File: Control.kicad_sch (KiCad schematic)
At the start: 25 parts, among them Q1 MMBT3904, U10 74AHC1G14GW, U11 74AHCT08PW, U12 74AHCT32PW, U13 74AHCT32PW, U15 74AHC1G14GW, U3 74AHCT00PW, U4 74AHC1G14GW, U6 74AHCT02PW, U7 74AHCT08PW, U9 74AHCT08PW

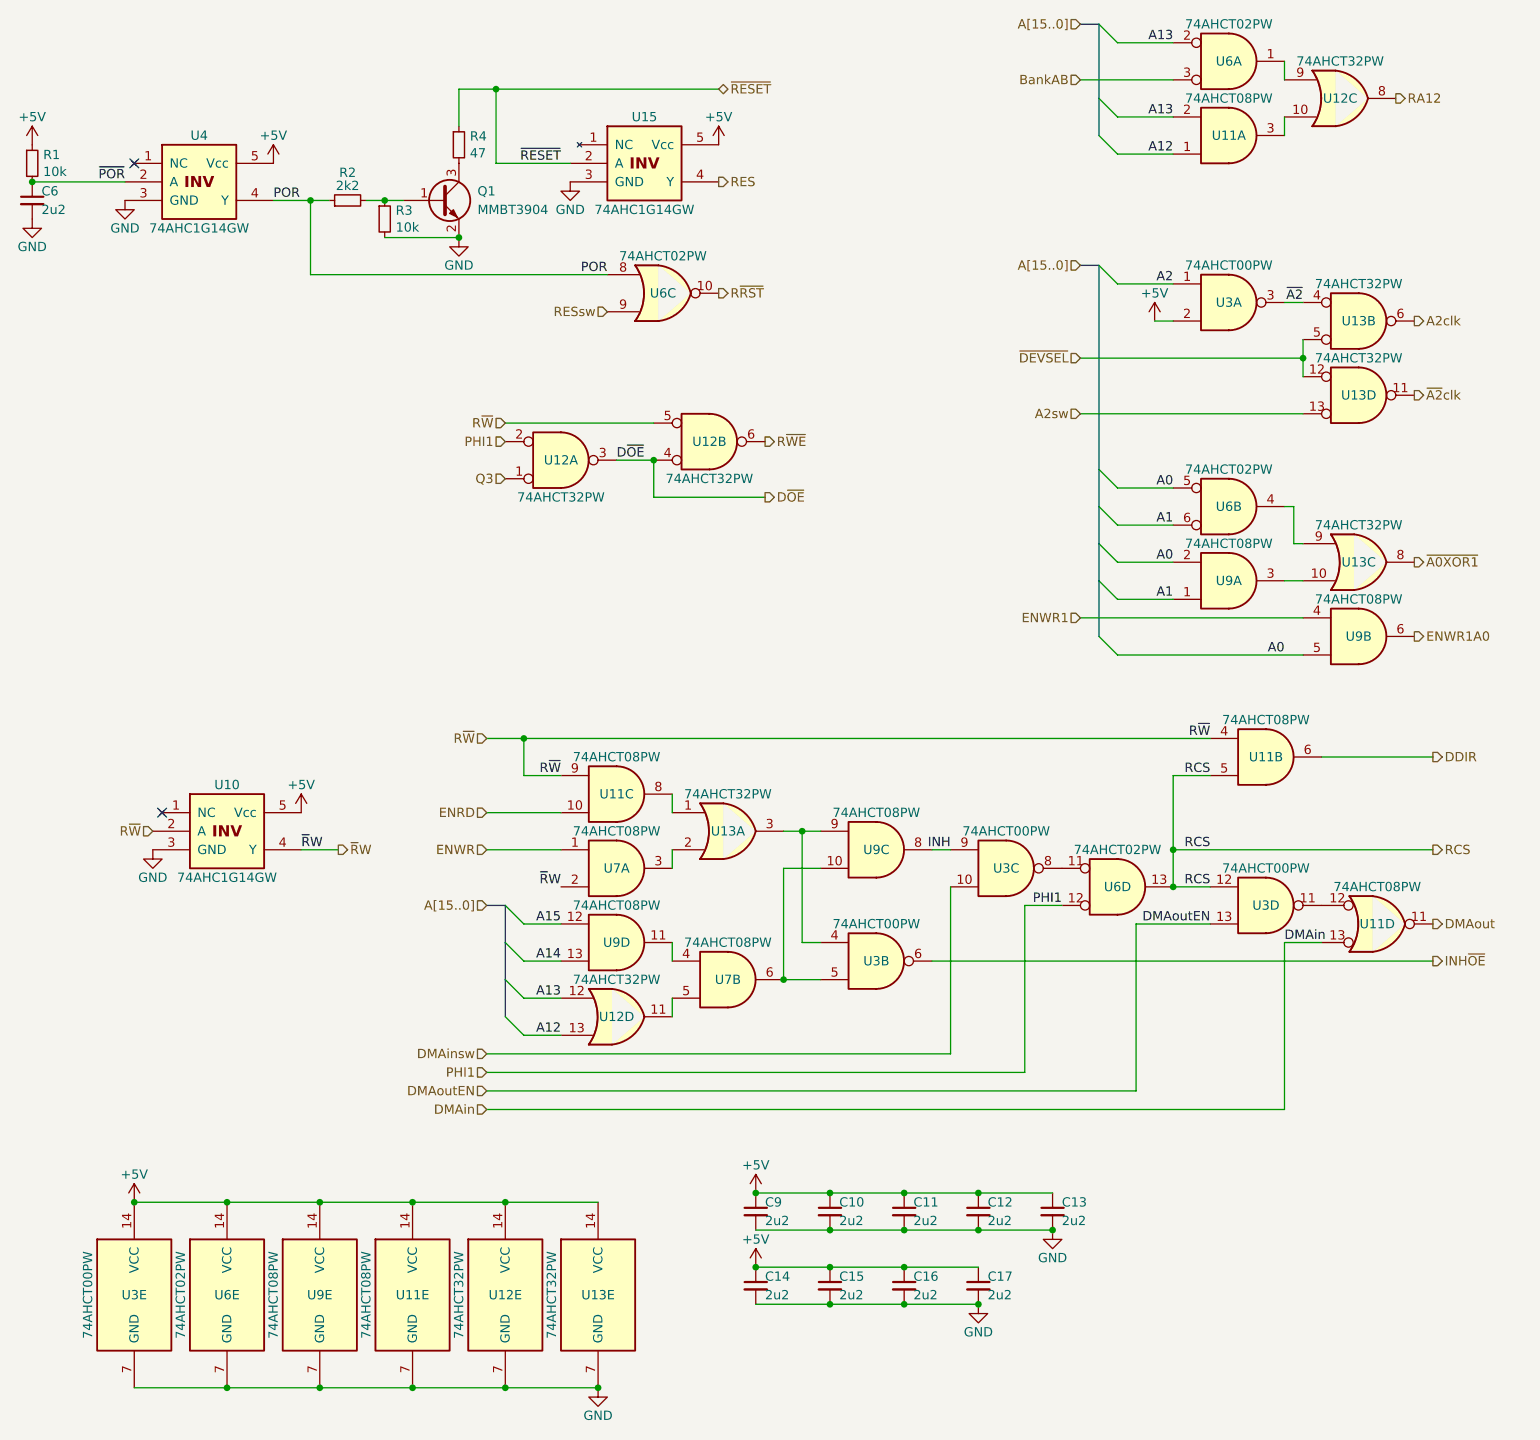
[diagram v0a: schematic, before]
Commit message: more
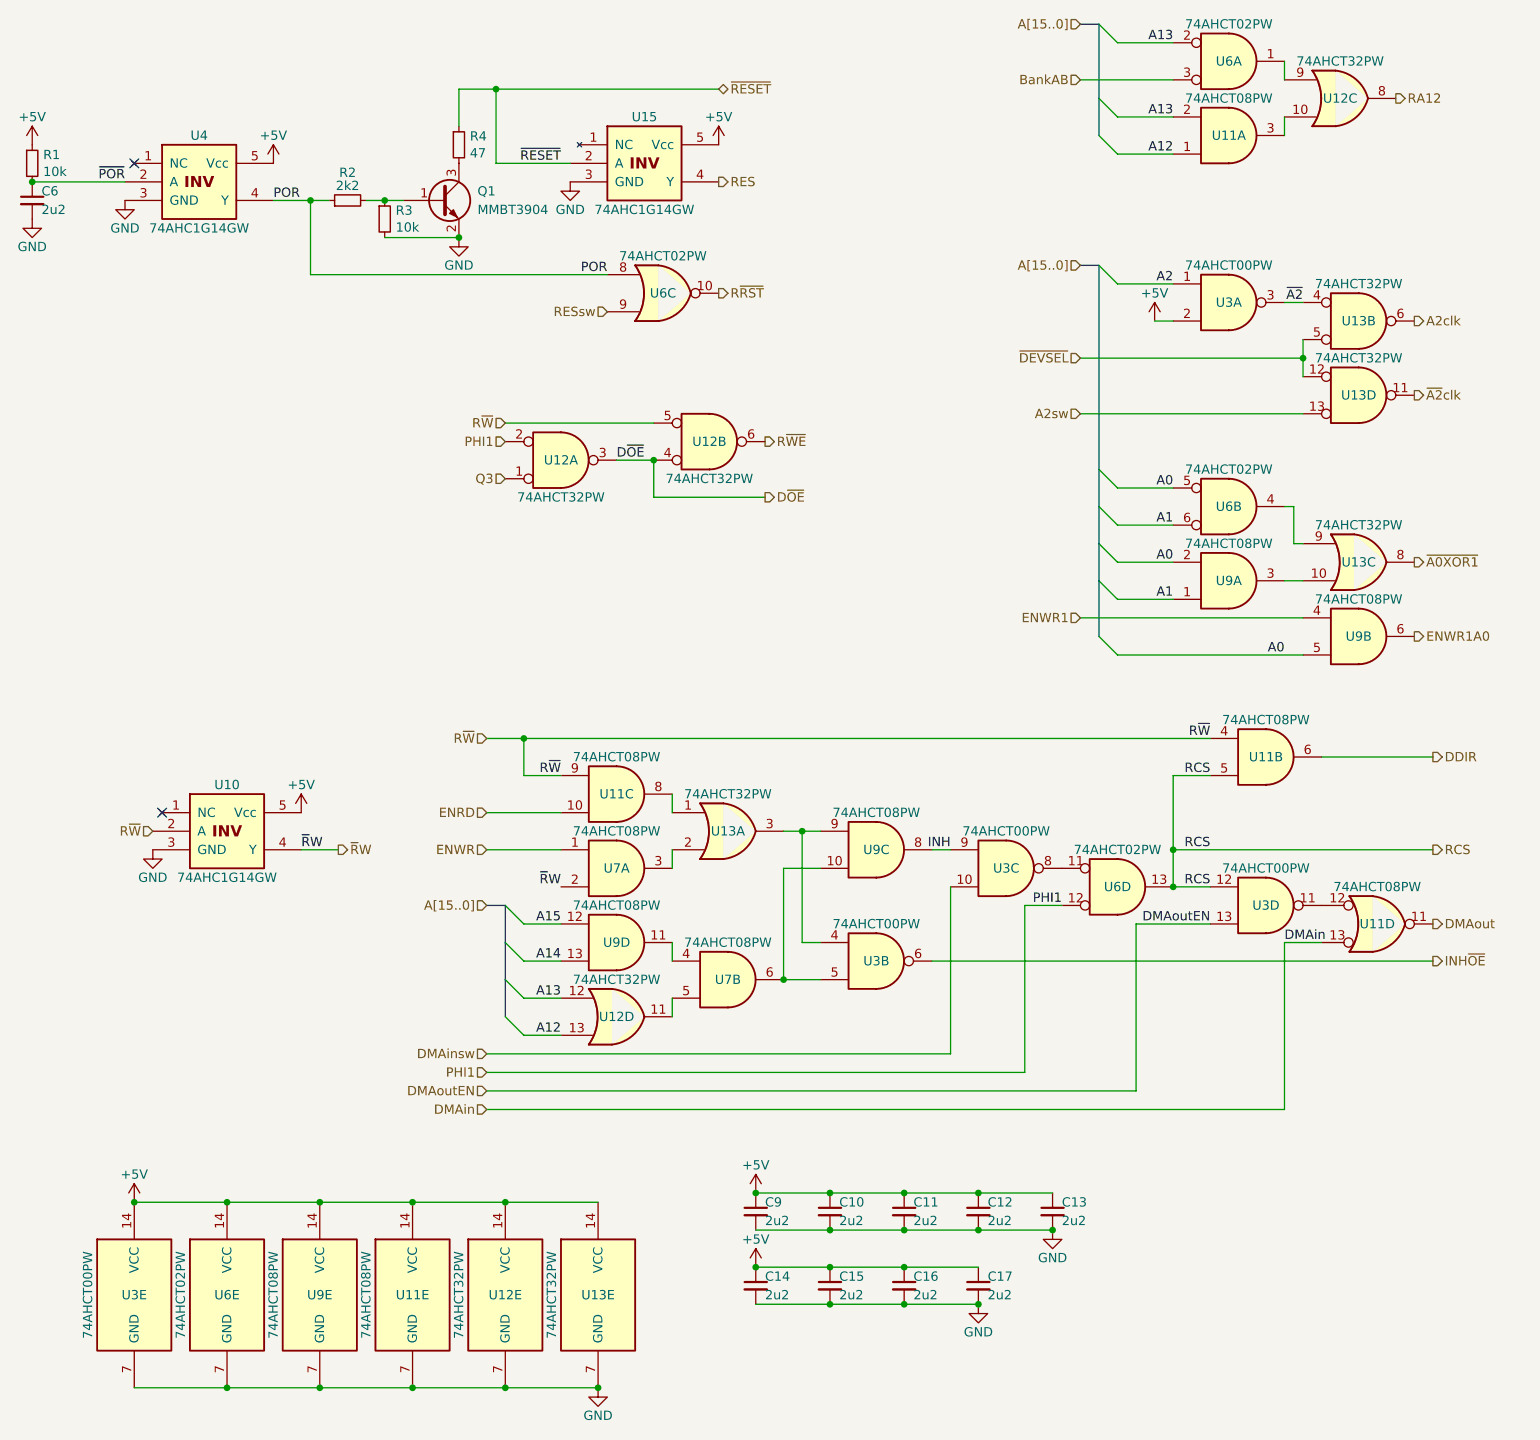
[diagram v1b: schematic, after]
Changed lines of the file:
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@@
 (kicad_sch
-	(version 20231120)
+	(version 20250114)
 	(generator "eeschema")
-	(generator_version "8.0")
+	(generator_version "9.0")
 	(paper "A4")
 	(title_block
@@
 	(label "A1"
 		(at 179.07 74.93 180)
-		(fields_autoplaced yes)
 		(effects
 			(font
@@
 	(label "A12"
 		(at 179.07 24.13 180)
-		(fields_autoplaced yes)
 		(effects
 			(font
@@
 	(label "INH"
 		(at 148.59 119.38 180)
-		(fields_autoplaced yes)
 		(effects
 			(font
@@
 	(label "D~{OE}"
 		(at 102.87 66.04 0)
-		(fields_autoplaced yes)
 		(effects
 			(font
@@
 	(label "A0"
 		(at 179.07 69.85 180)
-		(fields_autoplaced yes)
 		(effects
 			(font
@@
 	(label "~{RESET}"
 		(at 95.25 25.4 180)
-		(fields_autoplaced yes)
 		(effects
 			(font
@@
 	(label "A0"
 		(at 179.07 80.01 180)
-		(fields_autoplaced yes)
 		(effects
 			(font
@@
 	(label "DMAin"
 		(at 194.31 132.08 0)
-		(fields_autoplaced yes)
 		(effects
 			(font
@@
 	(label "A1"
 		(at 179.07 85.09 180)
-		(fields_autoplaced yes)
 		(effects
 			(font
@@
 	(label "DMAoutEN"
 		(at 184.15 129.54 180)
-		(fields_autoplaced yes)
 		(effects
 			(font
@@
 	(label "A0"
 		(at 194.31 92.71 180)
-		(fields_autoplaced yes)
 		(effects
 			(font
@@
 	(label "~{R}W"
 		(at 59.69 119.38 0)
-		(fields_autoplaced yes)
 		(effects
 			(font
@@
 	(label "POR"
 		(at 55.88 30.48 0)
-		(fields_autoplaced yes)
 		(effects
 			(font
@@
 	(label "POR"
 		(at 101.6 40.64 180)
-		(fields_autoplaced yes)
 		(effects
 			(font
@@
 	(label "~{A2}"
 		(at 196.85 44.45 180)
-		(fields_autoplaced yes)
 		(effects
 			(font
@@
 	(label "RCS"
 		(at 184.15 109.22 180)
-		(fields_autoplaced yes)
 		(effects
 			(font
@@
 	(label "~{R}W"
 		(at 95.25 124.46 180)
-		(fields_autoplaced yes)
 		(effects
 			(font
@@
 	(label "A2"
 		(at 179.07 41.91 180)
-		(fields_autoplaced yes)
 		(effects
 			(font
@@
 	(label "A13"
 		(at 179.07 8.89 180)
-		(fields_autoplaced yes)
 		(effects
 			(font
@@
 	(label "PHI1"
 		(at 163.83 127 180)
-		(fields_autoplaced yes)
 		(effects
 			(font
@@
 	(label "A13"
 		(at 95.25 139.7 180)
-		(fields_autoplaced yes)
 		(effects
 			(font
@@
 	(label "A13"
 		(at 179.07 19.05 180)
-		(fields_autoplaced yes)
 		(effects
 			(font
@@
 	(label "A15"
 		(at 95.25 129.54 180)
-		(fields_autoplaced yes)
 		(effects
 			(font
@@
 	(label "~{POR}"
 		(at 35.56 27.94 180)
-		(fields_autoplaced yes)
 		(effects
 			(font
@@
 	(label "A14"
 		(at 95.25 134.62 180)
-		(fields_autoplaced yes)
 		(effects
 			(font
@@
 	(label "R~{W}"
 		(at 184.15 104.14 180)
-		(fields_autoplaced yes)
 		(effects
 			(font
@@
 	(label "RCS"
 		(at 184.15 119.38 180)
-		(fields_autoplaced yes)
 		(effects
 			(font
@@
 	(label "A12"
 		(at 95.25 144.78 180)
-		(fields_autoplaced yes)
 		(effects
 			(font
@@
 	(label "RCS"
 		(at 184.15 124.46 180)
-		(fields_autoplaced yes)
 		(effects
 			(font
@@
 	(label "R~{W}"
 		(at 95.25 109.22 180)
-		(fields_autoplaced yes)
 		(effects
 			(font
@@
 		(shape output)
 		(at 212.09 46.99 0)
-		(fields_autoplaced yes)
 		(effects
 			(font
@@
 		(shape output)
 		(at 212.09 80.01 0)
-		(fields_autoplaced yes)
 		(effects
 			(font
@@
 		(shape input)
 		(at 166.37 13.97 180)
-		(fields_autoplaced yes)
 		(effects
 			(font
@@
 		(shape input)
 		(at 87.63 60.96 180)
-		(fields_autoplaced yes)
 		(effects
 			(font
@@
 		(shape input)
 		(at 166.37 6.35 180)
-		(fields_autoplaced yes)
 		(effects
 			(font
@@
 		(shape output)
 		(at 214.63 129.54 0)
-		(fields_autoplaced yes)
 		(effects
 			(font
@@
 		(shape input)
 		(at 87.63 63.5 180)
-		(fields_autoplaced yes)
 		(effects
 			(font
@@
 		(shape output)
 		(at 64.77 119.38 0)
-		(fields_autoplaced yes)
 		(effects
 			(font
@@
 		(shape input)
 		(at 85.09 119.38 180)
-		(fields_autoplaced yes)
 		(effects
 			(font
@@
 		(shape input)
 		(at 85.09 152.4 180)
-		(fields_autoplaced yes)
 		(effects
 			(font
@@
 		(shape input)
 		(at 166.37 87.63 180)
-		(fields_autoplaced yes)
 		(effects
 			(font
@@
 		(shape input)
 		(at 39.37 116.84 180)
-		(fields_autoplaced yes)
 		(effects
 			(font
@@
 		(shape input)
 		(at 166.37 39.37 180)
-		(fields_autoplaced yes)
 		(effects
 			(font
@@
 		(shape input)
 		(at 85.09 147.32 180)
-		(fields_autoplaced yes)
 		(effects
 			(font
@@
 		(shape input)
 		(at 87.63 68.58 180)
-		(fields_autoplaced yes)
 		(effects
 			(font
@@
 		(shape output)
 		(at 214.63 119.38 0)
-		(fields_autoplaced yes)
 		(effects
 			(font
@@
 		(shape output)
 		(at 116.84 43.18 0)
-		(fields_autoplaced yes)
 		(effects
 			(font
@@
 		(shape output)
 		(at 116.84 27.94 0)
-		(fields_autoplaced yes)
 		(effects
 			(font
@@
 		(shape output)
 		(at 123.19 63.5 0)
-		(fields_autoplaced yes)
 		(effects
 			(font
@@
 		(shape output)
 		(at 214.63 134.62 0)
-		(fields_autoplaced yes)
 		(effects
 			(font
@@
 		(shape output)
 		(at 212.09 57.15 0)
-		(fields_autoplaced yes)
 		(effects
 			(font
@@
 		(shape output)
 		(at 123.19 71.12 0)
-		(fields_autoplaced yes)
 		(effects
 			(font
@@
 		(shape output)
 		(at 209.55 16.51 0)
-		(fields_autoplaced yes)
 		(effects
 			(font
@@
 		(shape input)
 		(at 85.09 127 180)
-		(fields_autoplaced yes)
 		(effects
 			(font
@@
 		(shape input)
 		(at 85.09 104.14 180)
-		(fields_autoplaced yes)
 		(effects
 			(font
@@
 		(shape input)
 		(at 85.09 114.3 180)
-		(fields_autoplaced yes)
 		(effects
 			(font
@@
 		(shape input)
 		(at 101.6 45.72 180)
-		(fields_autoplaced yes)
 		(effects
 			(font
@@
 		(shape output)
 		(at 214.63 106.68 0)
-		(fields_autoplaced yes)
 		(effects
 			(font
@@
 		(shape input)
 		(at 85.09 149.86 180)
-		(fields_autoplaced yes)
 		(effects
 			(font
@@
 		(shape input)
 		(at 166.37 52.07 180)
-		(fields_autoplaced yes)
 		(effects
 			(font
@@
 		(shape input)
 		(at 85.09 154.94 180)
-		(fields_autoplaced yes)
 		(effects
 			(font
@@
 		(shape output)
 		(at 212.09 90.17 0)
-		(fields_autoplaced yes)
 		(effects
 			(font
@@
 		(shape input)
 		(at 166.37 59.69 180)
-		(fields_autoplaced yes)
 		(effects
 			(font
@@
 		(shape tri_state)
 		(at 116.84 15.24 0)
-		(fields_autoplaced yes)
-		(effects
-			(font
+		(effects
+			(font
